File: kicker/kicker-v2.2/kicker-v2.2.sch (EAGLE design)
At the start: 53 parts, among them IC1 7818TV, IC2 MCP601OT, J1 XT-60BATT_LABEL, Q1 IGB50N60T, Q3 IGB50N60T, U1 LT3750EMSPBF, U2 ATMEGA328P-AU

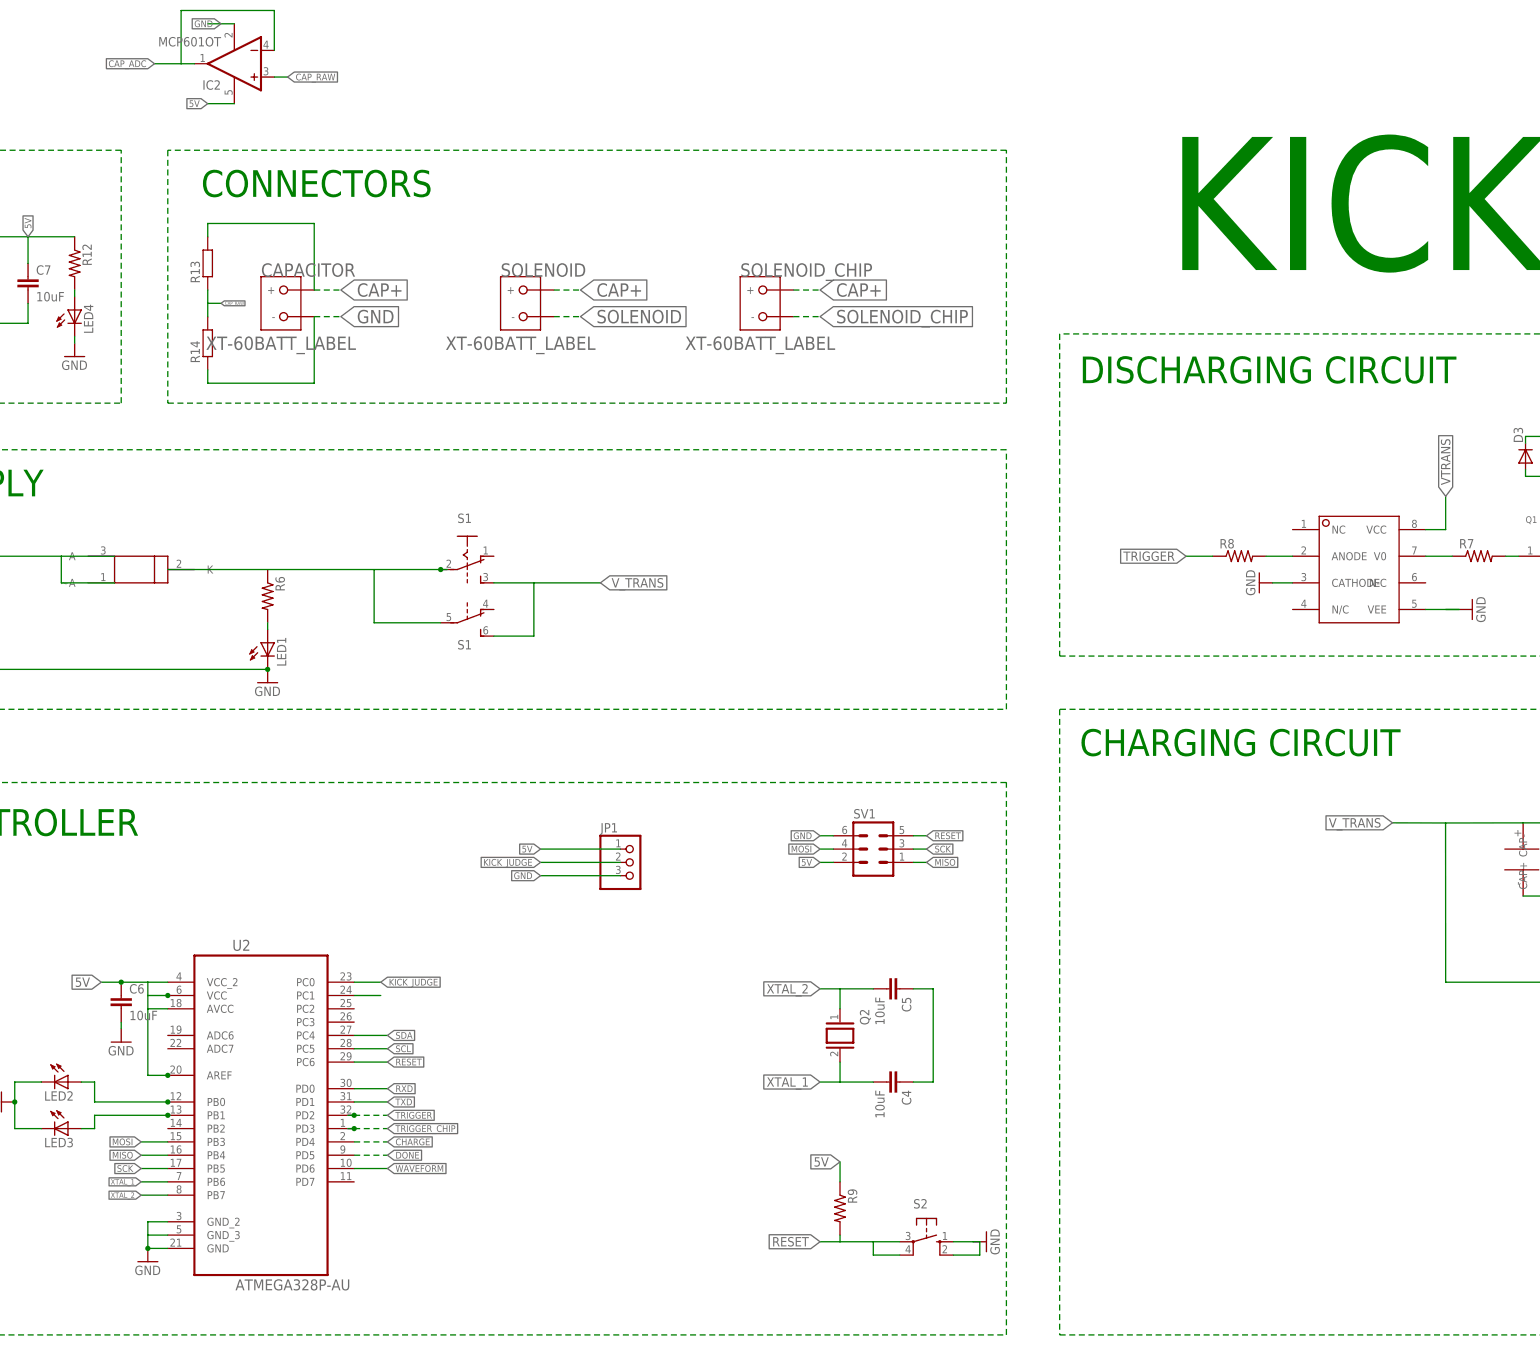
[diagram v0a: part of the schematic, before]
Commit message: Completed Circuit
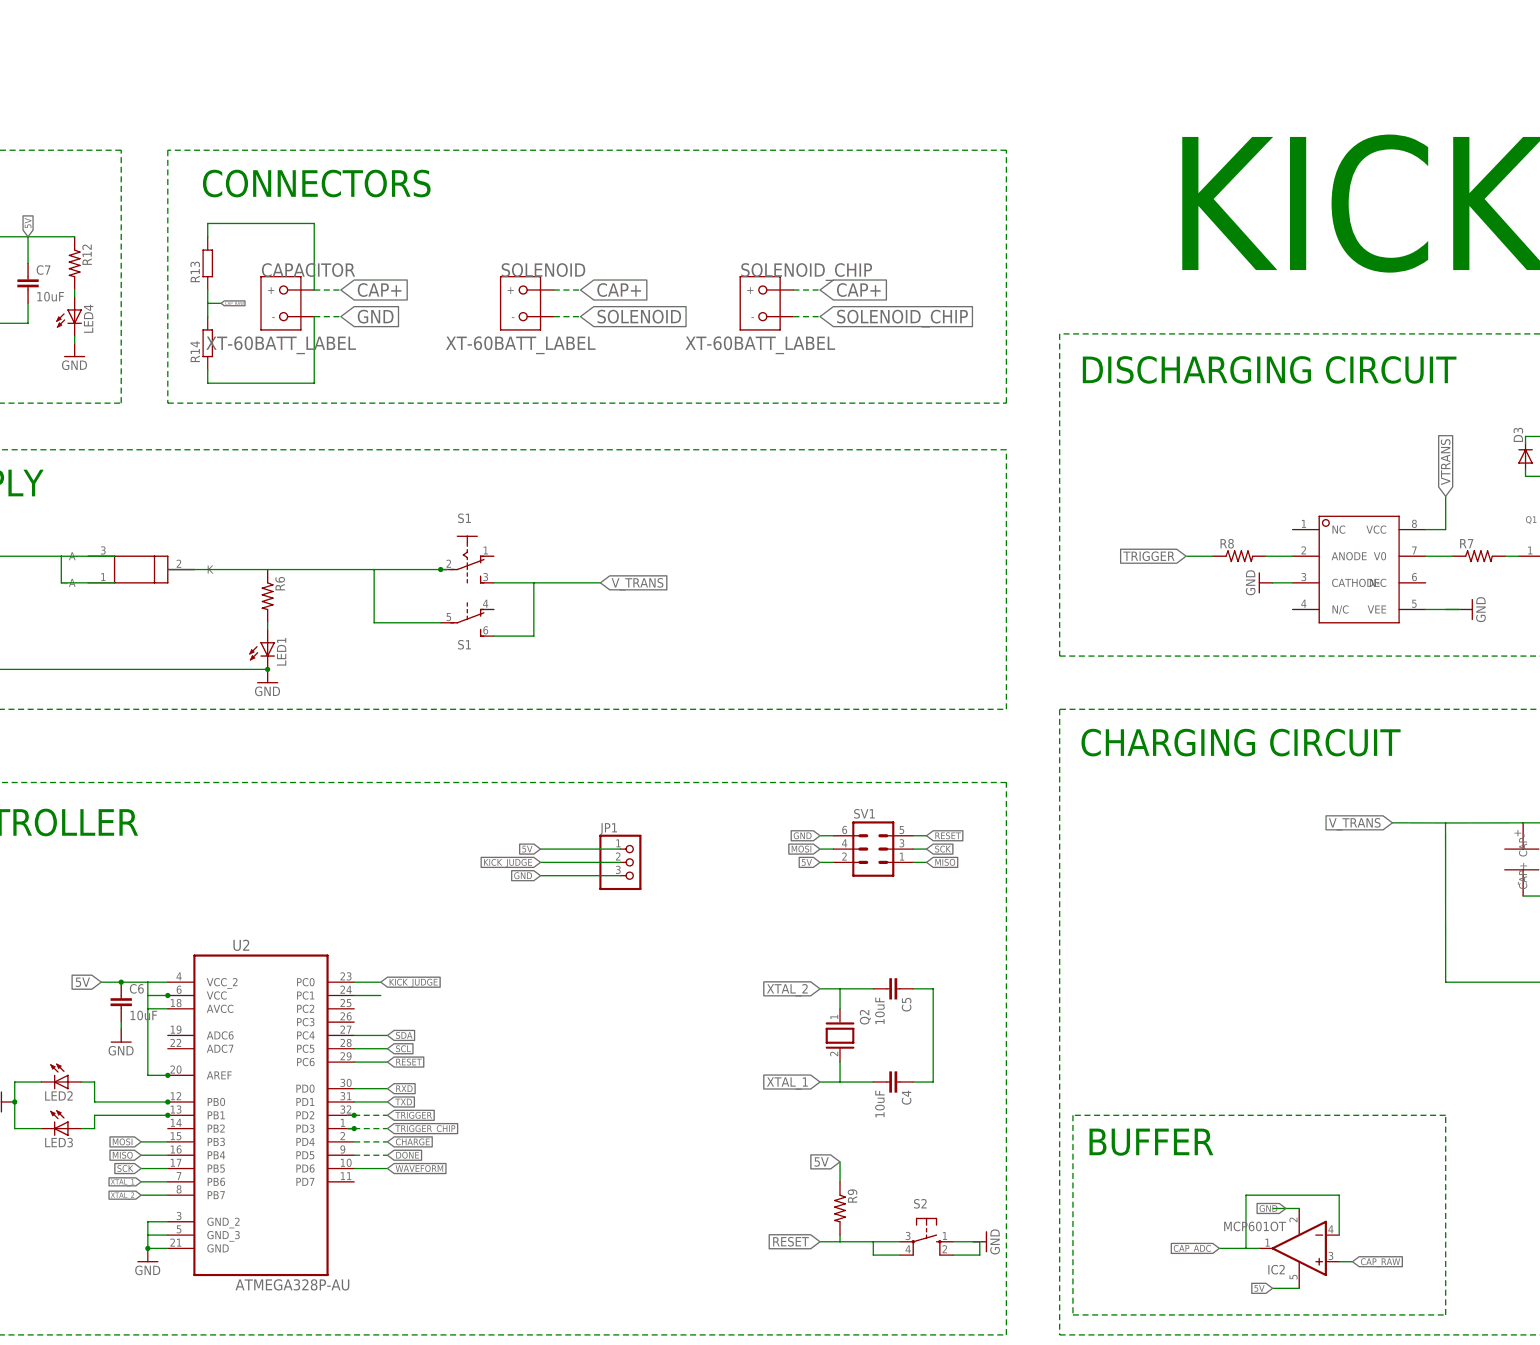
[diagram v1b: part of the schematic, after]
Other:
- note added: "BUFFER"
- moved on the sheet: IC2
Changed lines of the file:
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@@
 <text x="-123.19" y="111.76" size="5.08" layer="91">CONNECTORS</text>
 <text x="60.96" y="97.79" size="25.4" layer="91" font="fixed">KICKER 2018</text>
+<text x="45.72" y="-71.12" size="5.08" layer="91">BUFFER</text>
 </plain>
 <instances>
@@
 <instance part="R13" gate="G$1" x="-121.92" y="99.06" rot="R90"/>
 <instance part="R14" gate="G$1" x="-121.92" y="83.82" rot="R90"/>
-<instance part="IC2" gate="G$1" x="-116.84" y="137.16" rot="R180"/>
+<instance part="IC2" gate="G$1" x="86.36" y="-88.9" rot="R180"/>
 </instances>
 <busses>
@@
 <segment>
 <pinref part="IC2" gate="G$1" pin="V-"/>
-<wire x1="-116.84" y1="144.78" x2="-121.92" y2="144.78" width="0.1524" layer="91"/>
-<label x="-119.38" y="144.78" size="1.27" layer="95" rot="R180" xref="yes"/>
+<wire x1="86.36" y1="-81.28" x2="81.28" y2="-81.28" width="0.1524" layer="91"/>
+<label x="83.82" y="-81.28" size="1.27" layer="95" rot="R180" xref="yes"/>
 </segment>
 </net>
@@
 <segment>
 <pinref part="IC2" gate="G$1" pin="V+"/>
-<wire x1="-116.84" y1="129.54" x2="-121.92" y2="129.54" width="0.1524" layer="91"/>
-<label x="-121.92" y="129.54" size="1.27" layer="95" rot="R180" xref="yes"/>
+<wire x1="86.36" y1="-96.52" x2="81.28" y2="-96.52" width="0.1524" layer="91"/>
+<label x="81.28" y="-96.52" size="1.27" layer="95" rot="R180" xref="yes"/>
 </segment>
 </net>
@@
 <segment>
 <pinref part="IC2" gate="G$1" pin="+IN"/>
-<wire x1="-109.22" y1="134.62" x2="-106.68" y2="134.62" width="0.1524" layer="91"/>
-<label x="-106.68" y="134.62" size="1.27" layer="95" xref="yes"/>
+<wire x1="93.98" y1="-91.44" x2="96.52" y2="-91.44" width="0.1524" layer="91"/>
+<label x="96.52" y="-91.44" size="1.27" layer="95" xref="yes"/>
 </segment>
 </net>
@@
 <segment>
 <pinref part="IC2" gate="G$1" pin="-IN"/>
-<wire x1="-109.22" y1="139.7" x2="-109.22" y2="147.32" width="0.1524" layer="91"/>
-<wire x1="-109.22" y1="147.32" x2="-127" y2="147.32" width="0.1524" layer="91"/>
-<wire x1="-127" y1="147.32" x2="-127" y2="137.16" width="0.1524" layer="91"/>
+<wire x1="93.98" y1="-86.36" x2="93.98" y2="-78.74" width="0.1524" layer="91"/>
+<wire x1="93.98" y1="-78.74" x2="76.2" y2="-78.74" width="0.1524" layer="91"/>
+<wire x1="76.2" y1="-78.74" x2="76.2" y2="-88.9" width="0.1524" layer="91"/>
 <pinref part="IC2" gate="G$1" pin="OUT"/>
-<wire x1="-127" y1="137.16" x2="-124.46" y2="137.16" width="0.1524" layer="91"/>
-<wire x1="-127" y1="137.16" x2="-132.08" y2="137.16" width="0.1524" layer="91"/>
-<label x="-132.08" y="137.16" size="1.27" layer="95" rot="R180" xref="yes"/>
+<wire x1="76.2" y1="-88.9" x2="78.74" y2="-88.9" width="0.1524" layer="91"/>
+<wire x1="76.2" y1="-88.9" x2="71.12" y2="-88.9" width="0.1524" layer="91"/>
+<label x="71.12" y="-88.9" size="1.27" layer="95" rot="R180" xref="yes"/>
 </segment>
 <segment>
@@
 </segment>
 </net>
+<net name="N$6" class="0">
+<segment>
+<wire x1="43.18" y1="-63.5" x2="43.18" y2="-101.6" width="0.1524" layer="91" style="longdash"/>
+<wire x1="43.18" y1="-101.6" x2="114.3" y2="-101.6" width="0.1524" layer="91" style="longdash"/>
+<wire x1="114.3" y1="-101.6" x2="114.3" y2="-63.5" width="0.1524" layer="91" style="longdash"/>
+<wire x1="114.3" y1="-63.5" x2="43.18" y2="-63.5" width="0.1524" layer="91" style="longdash"/>
+</segment>
+</net>
